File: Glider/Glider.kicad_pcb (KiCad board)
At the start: 2 copper layers, 25 x 200 mm, 32 parts, among them J1 EuroPower, J2 OUT1, J3 IN1, J4 OUT2, J5 IN2, SW1 LIN/LOG, SW2 UP/DOWN, SW3 LIN/LOG, SW4 UP/DOWN, U1 TL082, U2 TL082

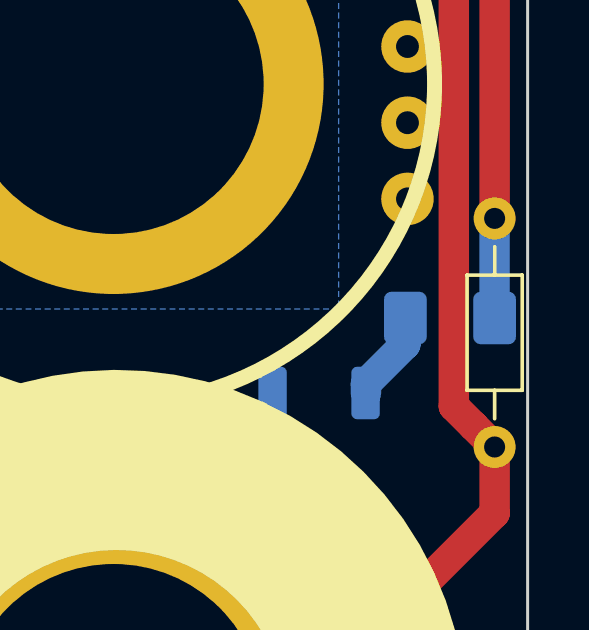
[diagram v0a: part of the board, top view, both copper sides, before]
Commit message: Prepared for release
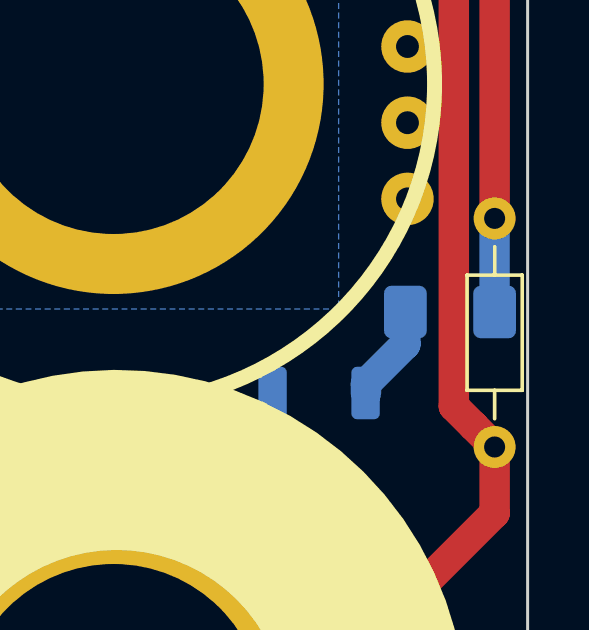
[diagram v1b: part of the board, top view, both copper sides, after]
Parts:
- moved R4 0.20 mm to (34.5, 182.7)
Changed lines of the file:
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@@
   )
   (setup
-    (last_trace_width 1.016)
+    (last_trace_width 0.1524)
     (user_trace_width 0.1524)
     (user_trace_width 0.254)
@@
   )
   (module Resistor_SMD:R_1206_3216Metric_Pad1.42x1.75mm_HandSolder (layer B.Cu)
-    (at 34.5125 182.9 180)
+    (at 34.5125 182.7 180)
     (descr "Resistor SMD 1206 (3216 Metric), square (rectangular) end terminal, IPC_7351 nominal with elongated pad for handsoldering. (Body size source: http://www.tortai-tech.com/upload/download/2011102023233369053.pdf), generated with kicad-footprint-generator")
     (tags "resistor handsolder")
